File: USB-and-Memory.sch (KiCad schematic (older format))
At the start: 1 part

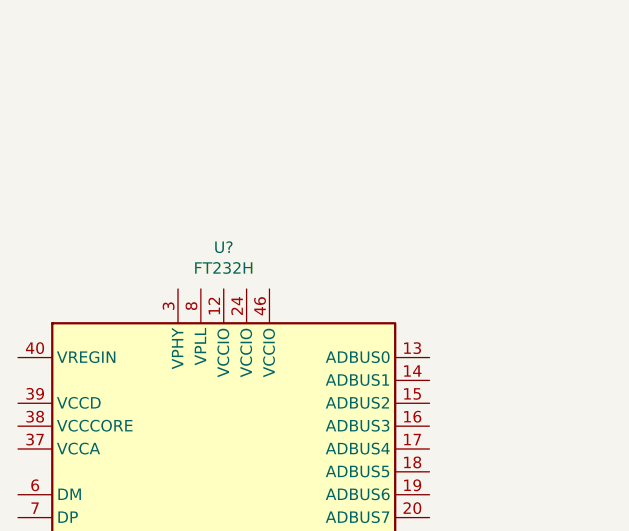
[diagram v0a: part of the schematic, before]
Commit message: More of the same
Signed-off-by: Eldalote <Eldalote.Electronics@gmail.com>
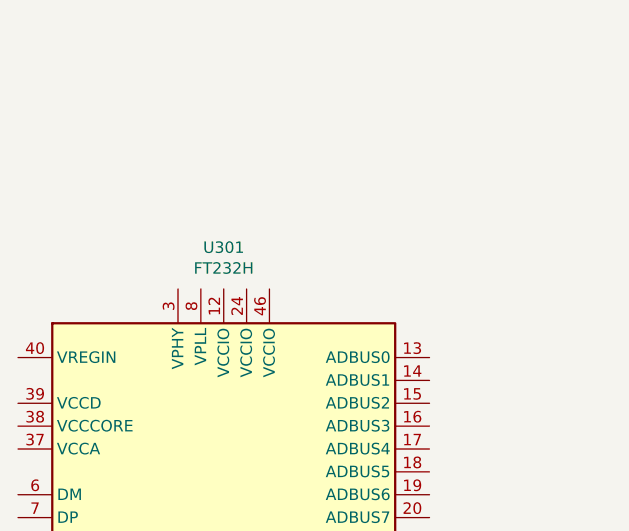
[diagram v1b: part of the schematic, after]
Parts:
- gave numbers to parts that had none: 1
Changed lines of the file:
@@
 USB: FTDI FT232H or FTDI FT232R\n\nMemory: Memory for FPGA bitstream data: MT25QL128ABA (non-JLC part)\n\nMemory: For FPGA user accessable data storage: W25Q128JVSIQ \n
 $Comp
-L Interface_USB:FT232H U?
+L Interface_USB:FT232H U301
 U 1 1 5F5894AD
 P 3000 3800
-F 0 "U?" H 3000 5481 50  0000 C CNN
+F 0 "U301" H 3000 5481 50  0000 C CNN
 F 1 "FT232H" H 3000 5390 50  0000 C CNN
 F 2 "Package_QFP:LQFP-48_7x7mm_P0.5mm" H 3000 3800 50  0001 C CNN
